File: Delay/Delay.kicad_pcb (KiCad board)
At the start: 2 copper layers, 192.7 x 104.5 mm, 186 parts, among them J101 Conn_02x08_Odd_Even, J102 AudioJack2_SwitchT, J103 AudioJack2_SwitchT, J104 AudioJack2_SwitchT, J105 AudioJack2_SwitchT, J106 AudioJack2_SwitchT, J107 AudioJack2_SwitchT, J108 AudioJack2_SwitchT, J201 AudioJack2_SwitchT, J301 AudioJack2_SwitchT, J401 AudioJack2_SwitchT, Q201 2N3904, Q301 2N3904, Q401 2N3904, SW101 SW_SPDT, SW102 SW_SPDT, U201 TL072, U202 TL072, U203 TL072, U204 PT2399, U301 TL072, U302 TL072, U303 TL072, U304 PT2399, U401 TL072, U402 TL072, U403 TL072, U404 PT2399

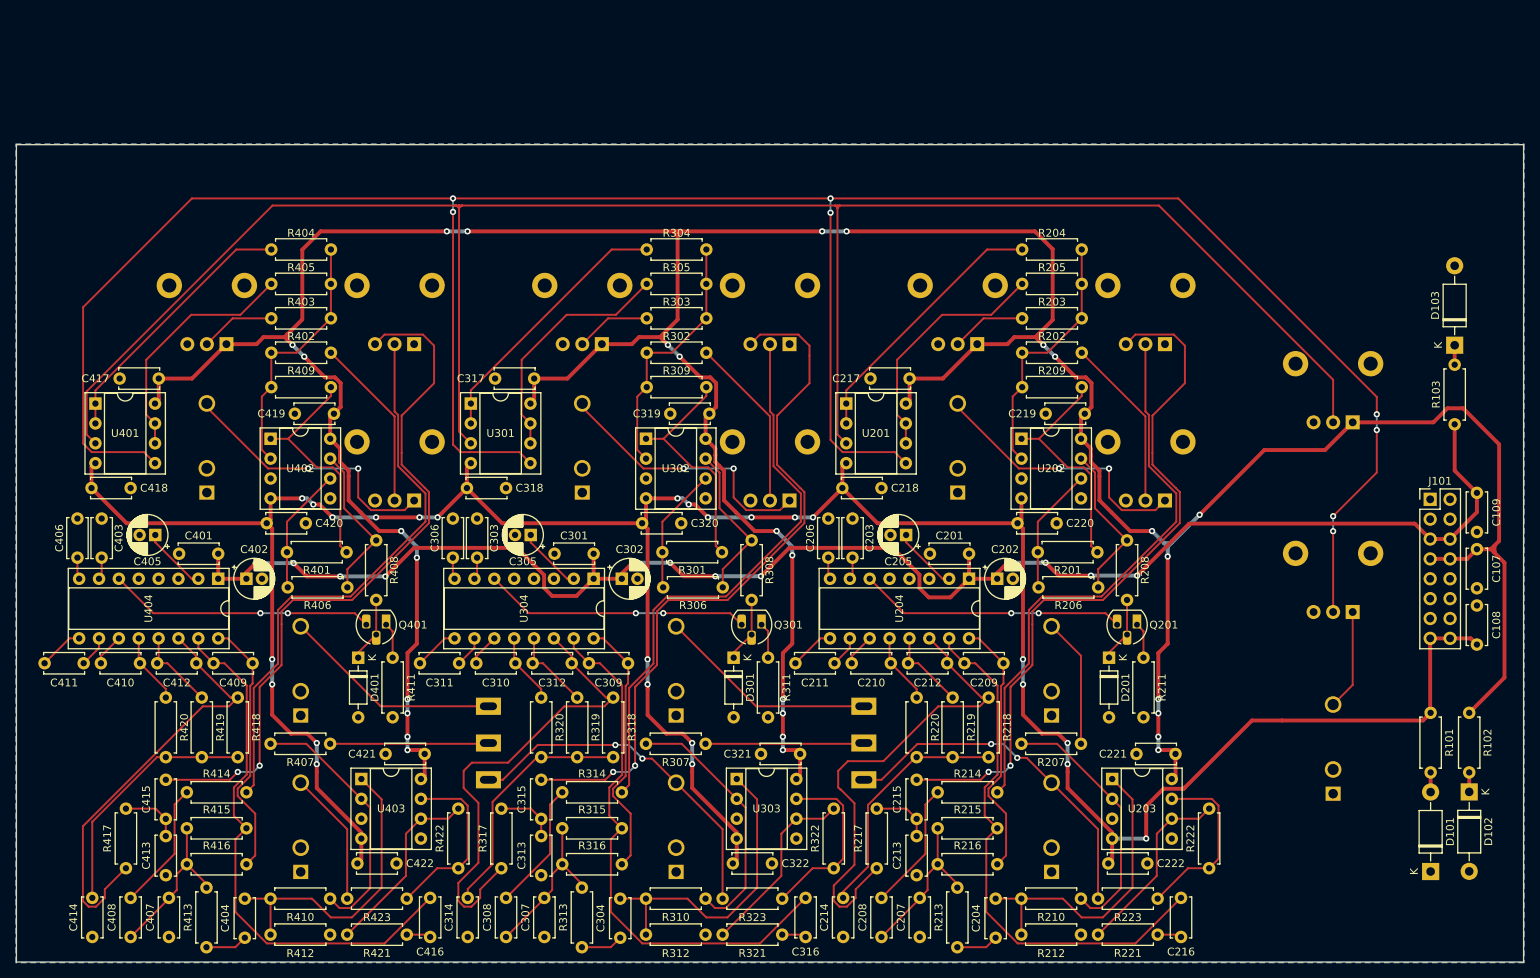
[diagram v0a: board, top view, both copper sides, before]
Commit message: Begin revised delay
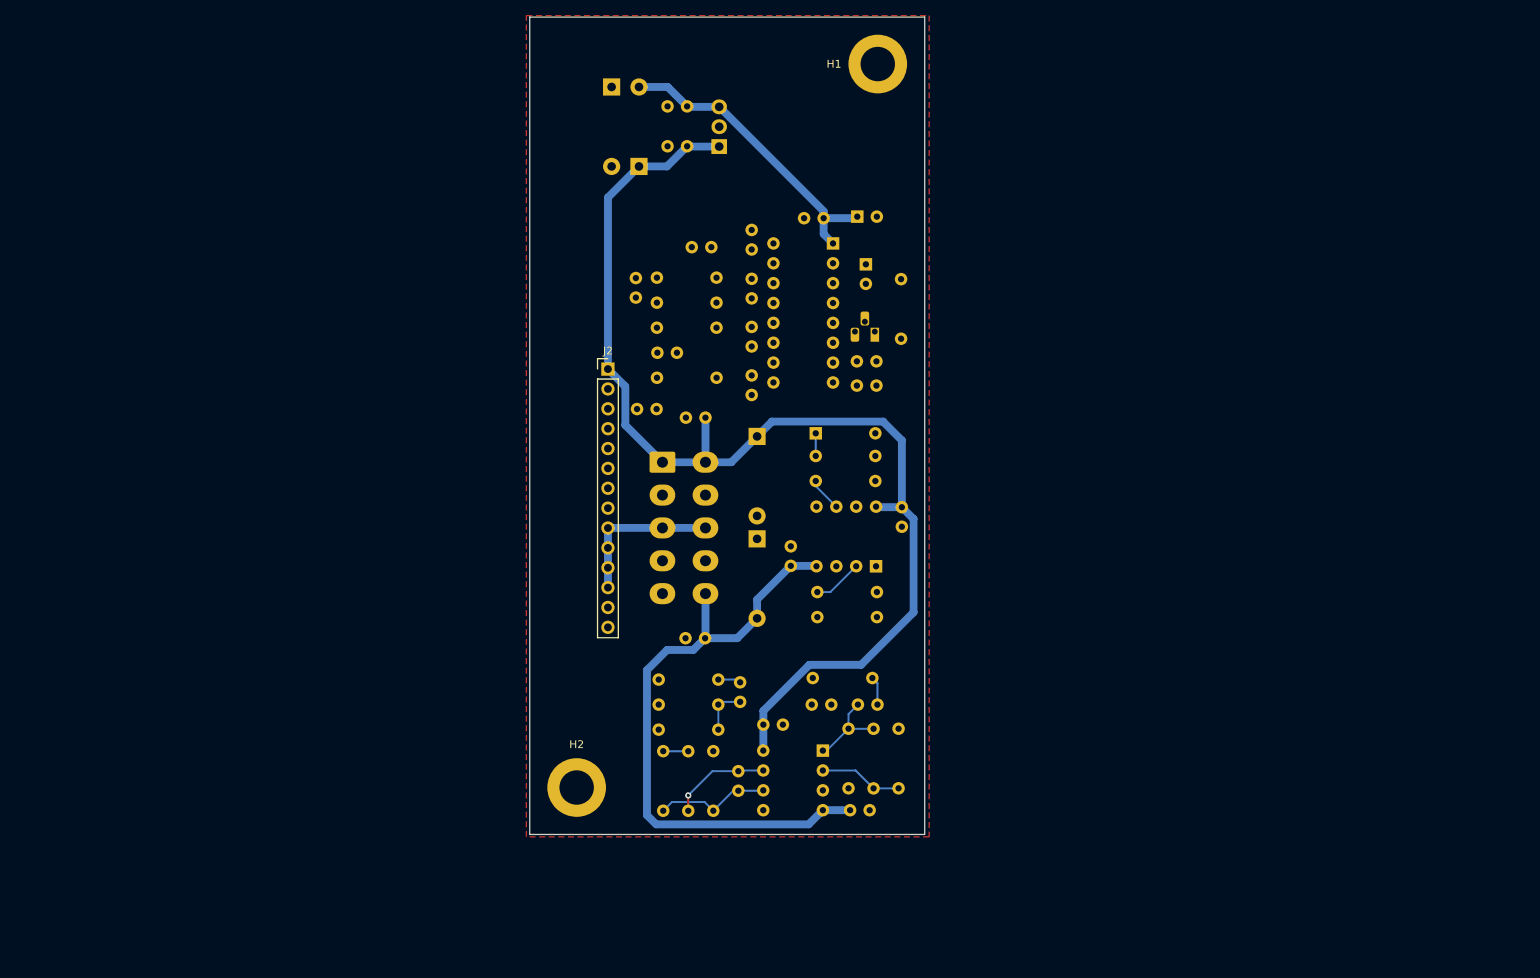
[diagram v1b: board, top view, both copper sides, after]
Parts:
- removed C107, C108, C109, C215, C216, C315, C316, C415, C416: 10u, Capacitor_THT:C_Disc_D5.0mm_W2.5mm_P5.00mm
- removed C201, C203, C206, C210, C211, C217, C218, C219, C220, C221, C222, C301, C303, C306, C310, C311, C317, C318, C319, C320, C321, C322, C401, C403, C406, C410, C411, C417, C418, C419, C420, C421, C422: 0.1u, Capacitor_THT:C_Disc_D5.0mm_W2.5mm_P5.00mm
- removed C202, C302, C402: 100u, Capacitor_THT:CP_Radial_D5.0mm_P2.00mm
- removed C204, C208, C304, C308, C404, C408: 4.7u, Capacitor_THT:C_Disc_D5.0mm_W2.5mm_P5.00mm
- removed C205, C305, C405: 47u, Capacitor_THT:CP_Radial_D5.0mm_P2.00mm
- removed C207, C214, C307, C314, C407, C414: 4.7n, Capacitor_THT:C_Disc_D5.0mm_W2.5mm_P5.00mm
- removed C209, C212, C309, C312, C409, C412: 680p, Capacitor_THT:C_Disc_D5.0mm_W2.5mm_P5.00mm
- removed C213, C313, C413: 10n, Capacitor_THT:C_Disc_D5.0mm_W2.5mm_P5.00mm
- removed D101, D102, D103: 1N5819, Diode_THT:D_DO-41_SOD81_P10.16mm_Horizontal
- removed D201, D301, D401: 1N4148, Diode_THT:D_DO-35_SOD27_P7.62mm_Horizontal
- removed J101: Conn_02x08_Odd_Even, Connector_PinHeader_2.54mm:PinHeader_2x08_P2.54mm_Vertical
- removed J102, J103, J104, J105, J106, J107, J108, J201, J301, J401: AudioJack2_SwitchT, Connector_Audio:Jack_3.5mm_QingPu_WQP-PJ398SM_Vertical_CircularHoles
- removed Q201, Q301, Q401: 2N3904, Package_TO_SOT_THT:TO-92_HandSolder
- removed R101, R102, R103: 10, Resistor_THT:R_Axial_DIN0207_L6.3mm_D2.5mm_P7.62mm_Horizontal
- removed R201, R206, R212, R301, R306, R312, R401, R406, R412: 100k, Resistor_THT:R_Axial_DIN0207_L6.3mm_D2.5mm_P7.62mm_Horizontal
- removed R202, R203, R204, R205, R208, R302, R303, R304, R305, R308, R402, R403, R404, R405, R408: 150k, Resistor_THT:R_Axial_DIN0207_L6.3mm_D2.5mm_P7.62mm_Horizontal
- removed R207, R217, R222, R307, R317, R322, R407, R417, R422: 5.6k, Resistor_THT:R_Axial_DIN0207_L6.3mm_D2.5mm_P7.62mm_Horizontal
- removed R209, R213, R218, R309, R313, R318, R409, R413, R418: 15k, Resistor_THT:R_Axial_DIN0207_L6.3mm_D2.5mm_P7.62mm_Horizontal
- removed R210, R221, R310, R321, R410, R421: 1.5k, Resistor_THT:R_Axial_DIN0207_L6.3mm_D2.5mm_P7.62mm_Horizontal
- removed R211, R223, R311, R323, R411, R423: 1k, Resistor_THT:R_Axial_DIN0207_L6.3mm_D2.5mm_P7.62mm_Horizontal
- removed R214, R314, R414: 8.2k, Resistor_THT:R_Axial_DIN0207_L6.3mm_D2.5mm_P7.62mm_Horizontal
- removed R215, R216, R219, R220, R315, R316, R319, R320, R415, R416, R419, R420: 10k, Resistor_THT:R_Axial_DIN0207_L6.3mm_D2.5mm_P7.62mm_Horizontal
- removed RV101, RV102, RV201, RV202, RV203, RV301, RV302, RV303, RV401, RV402, RV403: 50k, Potentiometer_THT:Potentiometer_Alpha_RD901F-40-00D_Single_Vertical_CircularHoles
- removed SW101, SW102: SW_SPDT, Custom:MTS-102_MTS-103_MTS-112_MTS-113_MTS-123
- removed U201, U202, U203, U301, U302, U303, U401, U402, U403: TL072, Package_DIP:DIP-8_W7.62mm_Socket
- removed U204, U304, U404: PT2399, Package_DIP:DIP-16_W7.62mm_Socket
- added C1: 10u, 0_Capacitor_THT:C_Disc_D5.5mm_W4.0mm_P2.50mm, B.Cu at (143.4, 72.4)
- added C10: 0.22u, 0_Capacitor_THT:C_Disc_D5.5mm_W2.5mm_P2.50mm, B.Cu at (141.1, 37.7)
- added C11: 0.1u, 0_Capacitor_THT:C_Disc_D5.5mm_W2.5mm_P2.50mm, B.Cu at (162.8, 68.3)
- added C12: 0.1u, 0_Capacitor_THT:C_Disc_D5.5mm_W2.5mm_P2.50mm, B.Cu at (150.8, 111.7)
- added C13: 0.1u, 0_Capacitor_THT:C_Disc_D5.5mm_W2.5mm_P2.50mm, B.Cu at (164.4, 122.6)
- added C14: 4.7n, 0_Capacitor_THT:C_Disc_D5.5mm_W2.5mm_P2.50mm, B.Cu at (157.0, 109.1)
- added C15: 4.7u, Capacitor_THT:C_Disc_D3.8mm_W2.6mm_P2.50mm, B.Cu at (147.8, 106.2)
- added C16: 0.1u, 0_Capacitor_THT:C_Disc_D5.5mm_W2.5mm_P2.50mm, B.Cu at (141.1, 32.6)
- added C17: 680p, 0_Capacitor_THT:C_Disc_D5.5mm_W2.5mm_P2.50mm, B.Cu at (149.3, 48.4)
- added C18: 0.1u, 0_Capacitor_THT:C_Disc_D5.5mm_W2.5mm_P2.50mm, B.Cu at (149.3, 60.8)
- added C19: 0.1u, 0_Capacitor_THT:C_Disc_D5.5mm_W2.5mm_P2.50mm, B.Cu at (149.3, 67.0)
- added C2: 10u, 0_Capacitor_THT:C_Disc_D5.5mm_W4.0mm_P2.50mm, B.Cu at (140.8, 100.6)
- added C20: 680p, 0_Capacitor_THT:C_Disc_D5.5mm_W2.5mm_P2.50mm, B.Cu at (149.3, 54.6)
- added C21: 10n, 0_Capacitor_THT:C_Disc_D5.5mm_W2.5mm_P2.50mm, B.Cu at (137.2, 64.1)
- added C22: 4.7n, 0_Capacitor_THT:C_Disc_D5.5mm_W2.5mm_P2.50mm, B.Cu at (134.5, 54.5)
- added C23: 10u, 0_Capacitor_THT:C_Disc_D5.5mm_W4.0mm_P2.50mm, B.Cu at (137.2, 71.3)
- added C24: 10u, 0_Capacitor_THT:C_Disc_D5.5mm_W4.0mm_P2.50mm, B.Cu at (144.2, 50.6)
- added C25: 10p, 0_Capacitor_THT:C_Disc_D5.5mm_W2.5mm_P2.50mm, B.Cu at (147.6, 117.6)
- added C3: 0.1u, 0_Capacitor_THT:C_Disc_D5.5mm_W2.5mm_P2.50mm, B.Cu at (158.5, 46.9)
- added C4: 100u, Capacitor_THT:CP_Radial_D6.3mm_P2.50mm, B.Cu at (162.8, 46.7)
- added C5: 0.1u, 0_Capacitor_THT:C_Disc_D5.5mm_W2.5mm_P2.50mm, B.Cu at (168.5, 83.8)
- added C6: 0.1u, 0_Capacitor_THT:C_Disc_D5.5mm_W2.5mm_P2.50mm, B.Cu at (154.3, 88.8)
- added C7: 0.1u, 0_Capacitor_THT:C_Disc_D5.5mm_W2.5mm_P2.50mm, B.Cu at (162.8, 65.2)
- added C8: 4.7u, Capacitor_THT:C_Disc_D3.8mm_W2.6mm_P2.50mm, B.Cu at (165.4, 109.1)
- added C9: 47u, Capacitor_THT:CP_Radial_D5.0mm_P2.50mm, B.Cu at (163.9, 52.8)
- added D1: 1N5819, Diode_THT:D_DO-41_SOD81_P10.16mm_Horizontal, B.Cu at (150.0, 74.8)
- added D2: 1N5819, Diode_THT:D_DO-41_SOD81_P10.16mm_Horizontal, B.Cu at (150.0, 87.9)
- added D3: 1N4148, Diode_THT:D_DO-35_SOD27_P7.62mm_Horizontal, B.Cu at (157.5, 74.4)
- added D4: 1N5819, Diode_THT:D_DO-41_SOD81_P10.16mm_Horizontal, B.Cu at (134.9, 40.3)
- added D5: 1N5819, Diode_THT:D_DO-41_SOD81_P10.16mm_Horizontal, B.Cu at (131.4, 30.1)
- added H1: MNT_STANDOFF, 0_MountingHole:MountingHole_Pitch7.5mm_Drill3.4mm, F.Cu at (165.4, 27.2)
- added H2: MNT_STANDOFF, 0_MountingHole:MountingHole_Pitch7.5mm_Drill3.4mm, F.Cu at (126.9, 119.7)
- added J1: Conn_02x05_Top_Bottom, Connector_Molex:Molex_Mini-Fit_Jr_5566-10A_2x05_P4.20mm_Vertical, B.Cu at (137.9, 78.1)
- added J2: Conn_01x14_Pin, Connector_PinHeader_2.54mm:PinHeader_1x14_P2.54mm_Vertical, F.Cu at (130.9, 66.2)
- added Q1: 2N3904, Package_TO_SOT_THT:TO-92_HandSolder, B.Cu at (165.1, 61.4)
- added R1: 100k, Resistor_THT:R_Axial_DIN0207_L6.3mm_D2.5mm_P7.62mm_Horizontal, B.Cu at (157.7, 97.9)
- added R10: 8.2k, Resistor_THT:R_Axial_DIN0207_L6.3mm_D2.5mm_P7.62mm_Horizontal, B.Cu at (145.0, 105.9)
- added R11: 10k, Resistor_THT:R_Axial_DIN0207_L6.3mm_D2.5mm_P7.62mm_Horizontal, B.Cu at (145.0, 109.1)
- added R12: 10k, Resistor_THT:R_Axial_DIN0207_L6.3mm_D2.5mm_P7.62mm_Horizontal, B.Cu at (145.0, 112.3)
- added R13: 5.6k, Resistor_THT:R_Axial_DIN0207_L6.3mm_D2.5mm_P7.62mm_Horizontal, B.Cu at (144.8, 67.3)
- added R14: 15k, Resistor_THT:R_Axial_DIN0207_L6.3mm_D2.5mm_P7.62mm_Horizontal, B.Cu at (144.8, 54.5)
- added R15: 10k, Resistor_THT:R_Axial_DIN0207_L6.3mm_D2.5mm_P7.62mm_Horizontal, B.Cu at (144.8, 57.7)
- added R16: 10k, Resistor_THT:R_Axial_DIN0207_L6.3mm_D2.5mm_P7.62mm_Horizontal, B.Cu at (144.8, 60.9)
- added R17: 1.5k, Resistor_THT:R_Axial_DIN0207_L6.3mm_D2.5mm_P7.62mm_Horizontal, B.Cu at (144.4, 115.0)
- added R18: 5.6k, Resistor_THT:R_Axial_DIN0207_L6.3mm_D2.5mm_P7.62mm_Horizontal, B.Cu at (138.0, 115.0)
- added R19: 1k, Resistor_THT:R_Axial_DIN0207_L6.3mm_D2.5mm_P7.62mm_Horizontal, B.Cu at (141.2, 115.0)
- added R2: 100k, Resistor_THT:R_Axial_DIN0207_L6.3mm_D2.5mm_P7.62mm_Horizontal, B.Cu at (165.1, 80.5)
- added R3: 5.6k, Resistor_THT:R_Axial_DIN0207_L6.3mm_D2.5mm_P7.62mm_Horizontal, B.Cu at (168.1, 112.2)
- added R4: 150k, Resistor_THT:R_Axial_DIN0207_L6.3mm_D2.5mm_P7.62mm_Horizontal, B.Cu at (157.5, 77.3)
- added R5: 15k, Resistor_THT:R_Axial_DIN0207_L6.3mm_D2.5mm_P7.62mm_Horizontal, B.Cu at (165.3, 94.7)
- added R6: 1.5k, Resistor_THT:R_Axial_DIN0207_L6.3mm_D2.5mm_P7.62mm_Horizontal, B.Cu at (164.9, 119.8)
- added R7: 1k, Resistor_THT:R_Axial_DIN0207_L6.3mm_D2.5mm_P7.62mm_Horizontal, B.Cu at (168.4, 62.3)
- added R8: 100k, Resistor_THT:R_Axial_DIN0207_L6.3mm_D2.5mm_P7.62mm_Horizontal, B.Cu at (161.7, 112.2)
- added R9: 15k, Resistor_THT:R_Axial_DIN0207_L6.3mm_D2.5mm_P7.62mm_Horizontal, B.Cu at (164.7, 105.7)
- added U1: TL072, Package_DIP:DIP-8_W7.62mm_Socket, B.Cu at (165.2, 91.4)
- added U2: TL072, Package_DIP:DIP-8_W7.62mm_Socket, B.Cu at (158.4, 115.0)
- added U3: PT2399, Package_DIP:DIP-16_W7.62mm, B.Cu at (159.7, 50.1)
- added U4: LM7805_TO220, Package_TO_SOT_THT:TO-220-3_Vertical, B.Cu at (145.2, 37.7)
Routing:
- net +12V: track 513.4 -> 148.6 mm, vias 29 -> 0
- net /Delay1/MasterTimeCV: track 323.3 -> 0.00 mm, vias 8 -> 0
- net -12V: track 363.9 -> 80.1 mm, vias 25 -> 0
- net /Delay1/MasterTime: track 255.0 -> 0.00 mm
- net +5V: track 205.9 -> 39.2 mm, vias 12 -> 0
- net Net-(C415-Pad2): track 91.7 -> 0.00 mm, vias 2 -> 0
- net Net-(C315-Pad2): track 91.7 -> 0.00 mm, vias 2 -> 0
- net Net-(C215-Pad2): track 91.7 -> 0.00 mm, vias 2 -> 0
- net Net-(R414-Pad2): track 72.8 -> 0.00 mm
- net Net-(R314-Pad2): track 72.8 -> 0.00 mm
- net Net-(R214-Pad2): track 72.8 -> 0.00 mm
- net Net-(C209-Pad2): track 69.3 -> 0.00 mm
- net Net-(C409-Pad2): track 69.3 -> 0.00 mm
- net Net-(C309-Pad2): track 69.3 -> 0.00 mm
- net Net-(C212-Pad1): track 61.5 -> 0.00 mm
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- added copper zone on F.Cu, net GND
- removed copper zone on B.Cu, net GND
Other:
- board size 192.7 x 104.5 mm -> 50.5 x 104.5 mm
